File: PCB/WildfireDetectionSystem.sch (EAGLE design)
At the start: 61 parts, among them IC1 STM32L476RGT6, J1 10118192-0001LF, J3 B4B-XH-A, J4 B5B-XH-A, SW1 1825910-6, U1 BME280, U2 LD39050PU33R, U3 NEO-6M-GPS, U4 24AA32A-I/MS, Y1 ABLS-8.000MHZ-B2-T, Y2 ECS-.327-12.5-12QS-TR

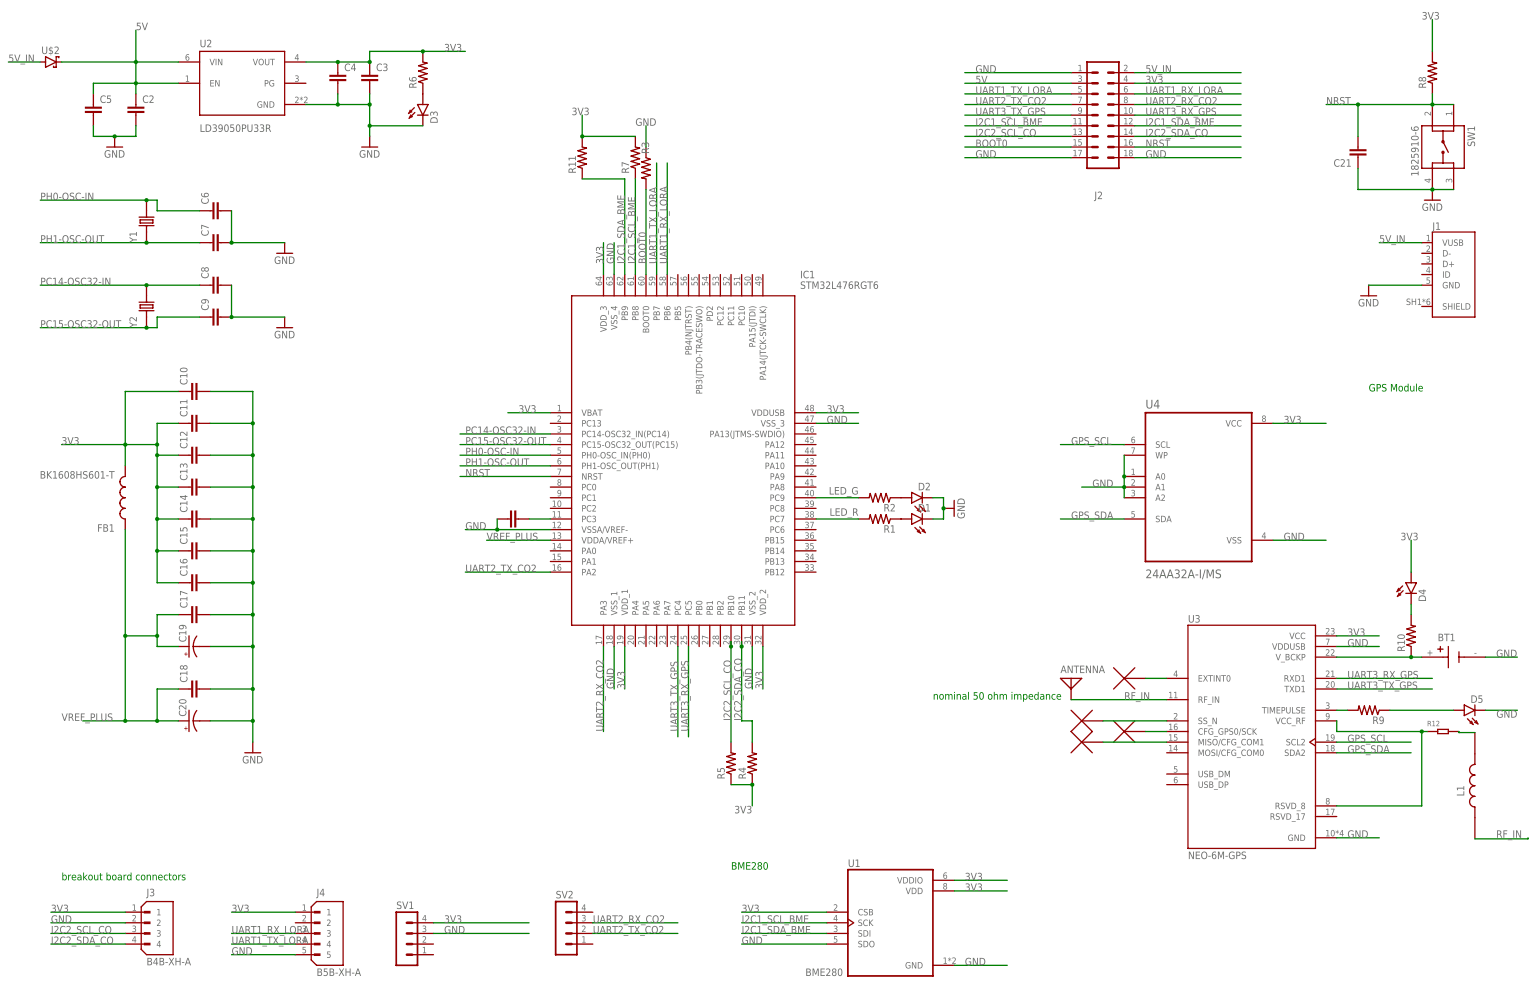
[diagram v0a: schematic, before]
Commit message: board and schematic changes
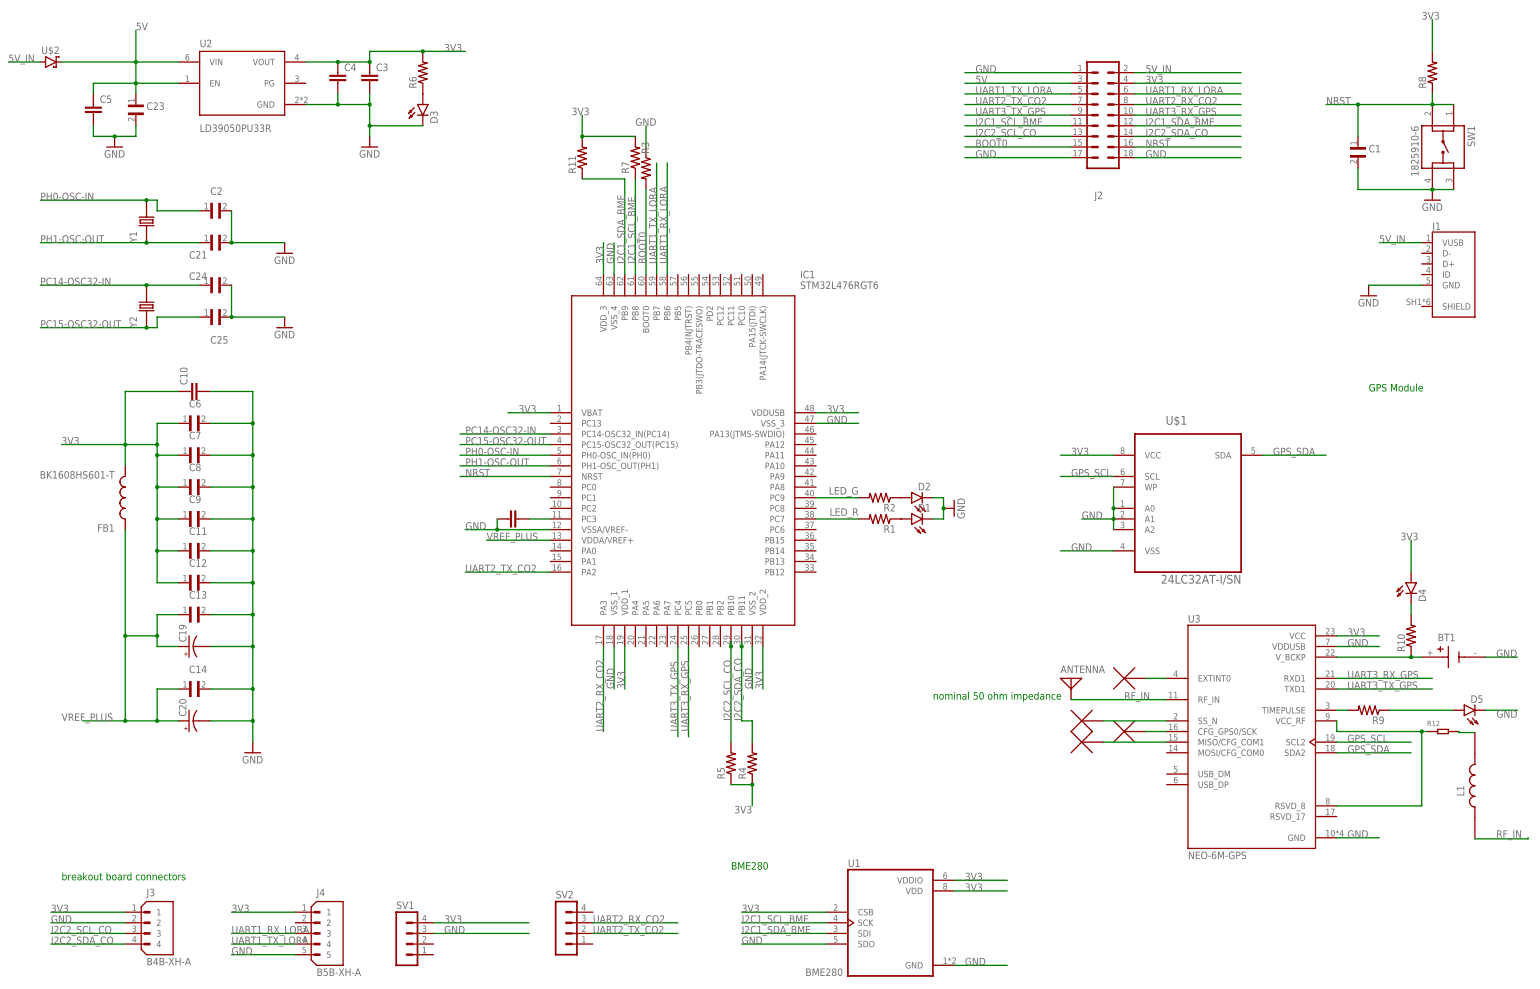
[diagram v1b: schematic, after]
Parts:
- removed C15, C16, C17, C18: CC0402KRX7R7BB104, ce-capstone:CC0402KRX7R7BB104
- removed U4: 24AA32A-I/MS, 24AA32A-I_MS:24AA32A-I/MS
- added C1, C23: CL05B104KO5NNNC, CL05B104KO5NNNC:CL05B104KO5NNNC
- added C24, C25: CL10C200JB8NNNC, CL10C200JB8NNNC:CL10C200JB8NNNC
- added U$1: 24LC32AT-I/SN, 24LC32AT-I_SN:24LC32AT-I/SN
- C11, C12, C13, C14: value CC0402KRX7R7BB104 -> CL05B104KO5NNNC; device ce-capstone:CC0402KRX7R7BB104 -> CL05B104KO5NNNC:CL05B104KO5NNNC
- C2, C21: value CC0402KRX7R7BB104 -> CL10C200JB8NNNC; device ce-capstone:CC0402KRX7R7BB104 -> CL10C200JB8NNNC:CL10C200JB8NNNC
- C6, C7, C8, C9: value CC0402JRNPO9BN200 -> CL05B104KO5NNNC; device ce-capstone:CC0402JRNPO9BN200 -> CL05B104KO5NNNC:CL05B104KO5NNNC
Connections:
- net 3V3: now also C6.1, C7.1, C8.1, C9.1, U$1.VCC; no longer C13.1, C14.1, C15.1, C16.1, U4.VCC
- net 5V: now also C23.1; no longer C2.1
- net GND: now also C1.2, C21.2, C23.2, C24.2, C25.2, U$1.A0, U$1.A1, U$1.A2, U$1.VSS, U$1.WP; no longer C15.2, C16.2, C17.2, C18.2, C21.1, U4.A0, U4.A1, U4.A2, U4.VSS, U4.WP
- net GPS_SCL: now also U$1.SCL; no longer U4.SCL
- net GPS_SDA: now also U$1.SDA; no longer U4.SDA
- net NRST: now also C1.1; no longer C21.2
- net PC14-OSC32-IN: now also C24.1; no longer C8.1
- net PC15-OSC32-OUT: now also C25.1; no longer C9.1
- net PH0-OSC-IN: now also C2.1; no longer C6.1
- net PH1-OSC-OUT: now also C21.1; no longer C7.1
- net VREF_PLUS: now also C13.1, C14.1; no longer C17.1, C18.1
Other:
- moved on the sheet: C11, C12, C13, C14, C2, C21, C6, C7, C8, C9
